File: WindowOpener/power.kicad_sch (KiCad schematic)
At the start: 8 parts, among them J3 Batt_Conn1, J4 Batt_Conn2, U3 AZ1117CH2-3.3

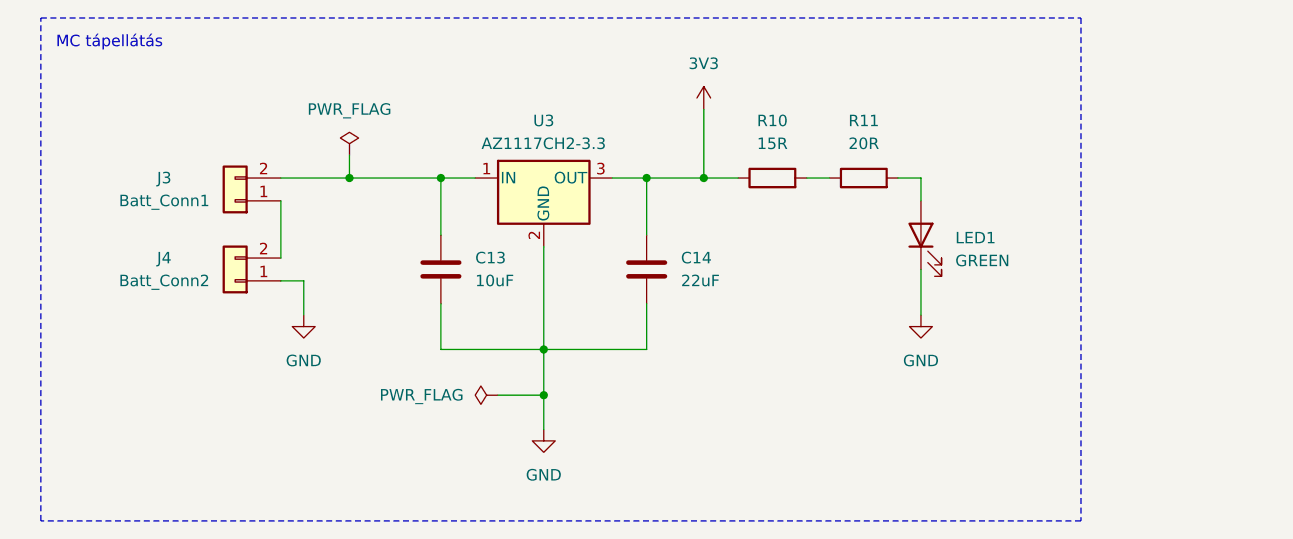
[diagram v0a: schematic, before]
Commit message: v0.1
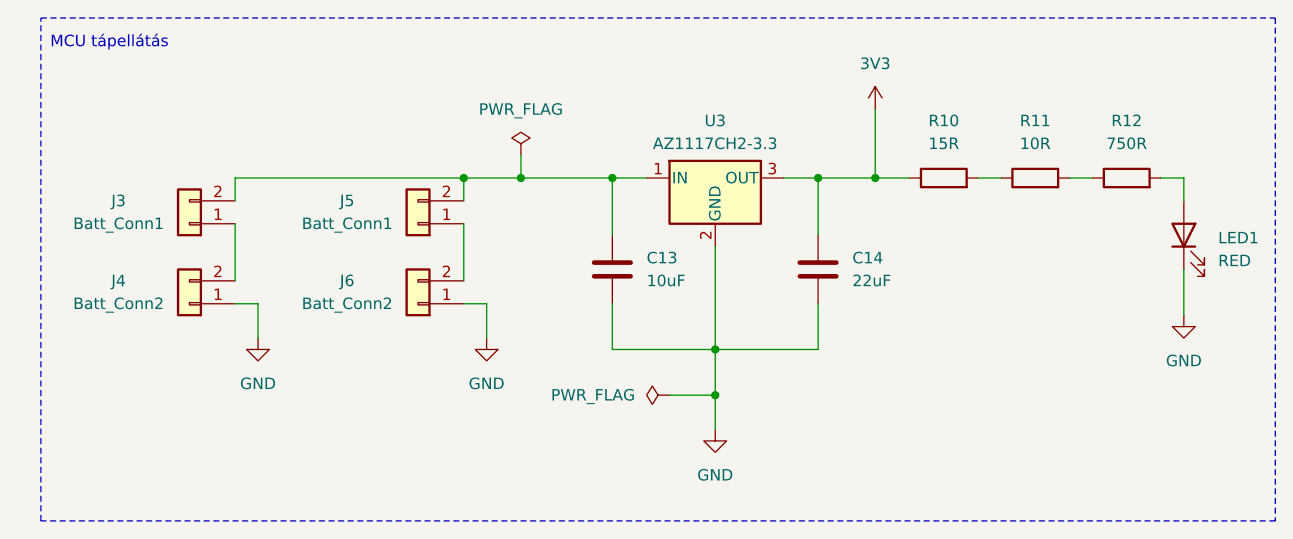
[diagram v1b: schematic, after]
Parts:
- added J5: Batt_Conn1, Battery:BatteryHolder_Keystone_1042_1x18650, symbol Connector_Generic:Conn_01x02
- added J6: Batt_Conn2, Battery:BatteryHolder_Keystone_1042_1x18650, symbol Connector_Generic:Conn_01x02
- added R12: 750R, LED_SMD:LED_1206_3216Metric_Pad1.42x1.75mm_HandSolder, symbol Device:R
- LED1: value GREEN -> RED; footprint SmartHomeFootprints:LED_1411 -> LED_SMD:LED_1206_3216Metric_Pad1.42x1.75mm_HandSolder; Store link https://hu.farnell.com/multicomp-pro/mp005918/led-green-225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 -> https://hu.farnell.com/kingbright/kptd-3216lvsurck/chip-led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
- R11: value 20R -> 10R; footprint Resistor_SMD:R_1210_3225Metric_Pad1.30x2.65mm_HandSolder -> LED_SMD:LED_1206_3216Metric_Pad1.42x1.75mm_HandSolder; Store link https://hu.farnell.com/vishay/crcw121020r0fkea/res-20r-1-0-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 -> https://hu.farnell.com/panasonic/erj8geyj100v/res-10r-5-0-2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
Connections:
- net GND: now also J6.1 (Pin_1)
- net at R11.2: now also R12.1; no longer LED1.2 (A)
- net at C13.1, J3.2 (Pin_2), U3.1 (IN): now also J5.2 (Pin_2)
- new net: J5.1 (Pin_1), J6.2 (Pin_2)
- new net: LED1.2 (A), R12.2
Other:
- note added: "MCU tápellátás"
- note removed: "MC tápellátás"
- moved on the sheet: C13, C14, J3, J4, LED1, R10, R11, U3
